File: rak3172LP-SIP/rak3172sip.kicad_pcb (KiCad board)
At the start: 2 copper layers, 46.5 x 29 mm, 46 parts, among them J1 U.FL, J2 Conn_ARM_SWD_TagConnect_TC203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, J4 Conn_01x03_Socket, J5 Conn_01x02_Socket, J6 Conn_01x08_Socket, U1 RAK3172-SIP

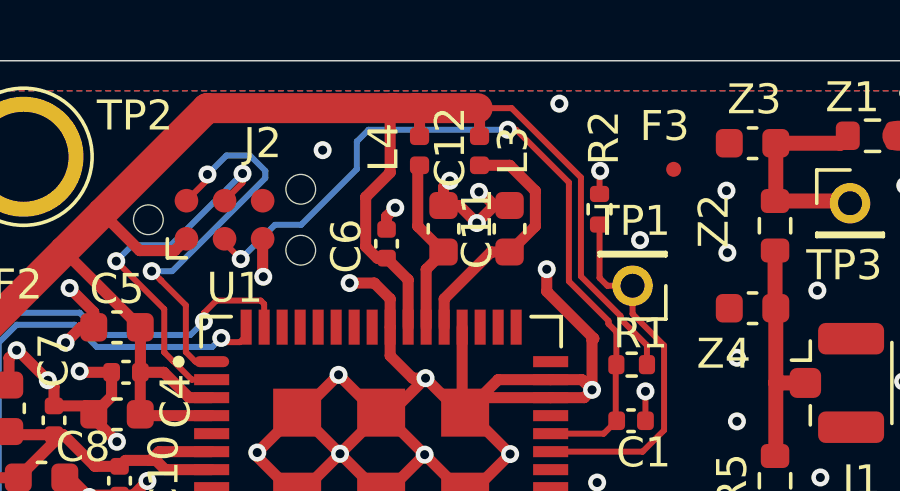
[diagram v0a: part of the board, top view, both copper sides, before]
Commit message: 0v02
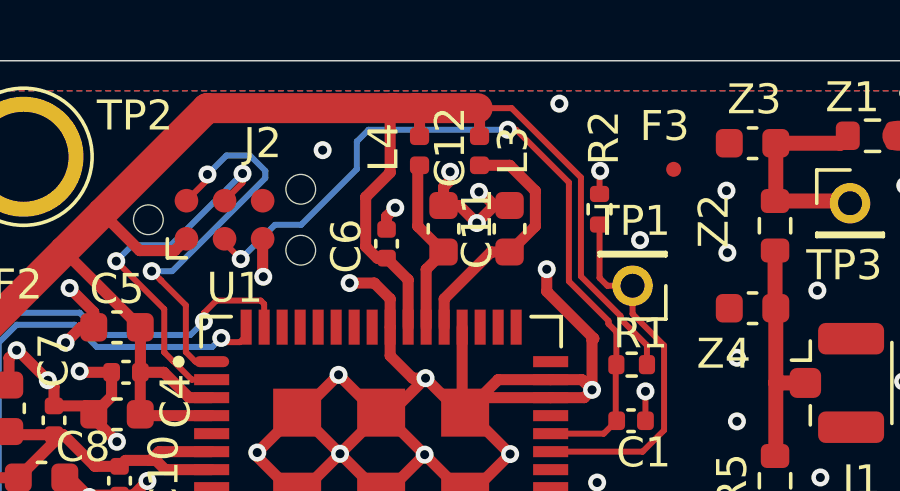
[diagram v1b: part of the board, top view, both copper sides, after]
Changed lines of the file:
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@@
 			(outputformat 1)
 			(mirror no)
-			(drillshape 1)
+			(drillshape 0)
 			(scaleselection 1)
-			(outputdirectory "")
+			(outputdirectory "rak3172_prod/")
 		)
 	)
@@
 		(sheetname "/")
 		(sheetfile "rak3172sip.kicad_sch")
-		(attr smd)
+		(attr smd dnp)
 		(fp_line
 			(start -0.237258 -0.5225)
@@
 		(sheetname "/")
 		(sheetfile "rak3172sip.kicad_sch")
-		(attr smd)
+		(attr smd dnp)
 		(fp_line
 			(start -0.237258 -0.5225)
@@
 			)
 		)
-		(property "Description" "Inductor with ferrite core, small symbol"
+		(property "Description" "FerriteBead Murata MPZ1005S121ETD25"
 			(at 0 0 0)
 			(layer "F.Fab")
@@
 		(sheetname "/")
 		(sheetfile "rak3172sip.kicad_sch")
-		(attr smd)
+		(attr smd dnp)
 		(fp_line
 			(start -0.14058 0.51)
@@
 			)
 		)
-		(property "Description" "Inductor with ferrite core, small symbol"
+		(property "Description" "FerriteBead Murata MPZ1005S121ETD25"
 			(at 0 0 90)
 			(layer "F.Fab")
@@
 			)
 		)
-		(property "Description" "Inductor"
+		(property "Description" "Inductor LQM21DN150M70L"
 			(at 0 0 90)
 			(layer "F.Fab")
@@
 		(sheetname "/")
 		(sheetfile "rak3172sip.kicad_sch")
-		(attr through_hole)
+		(attr through_hole exclude_from_bom)
 		(fp_line
 			(start -1.38 6.46)
@@
 			)
 		)
-		(property "Description" "Inductor with ferrite core, small symbol"
+		(property "Description" "FerriteBead Murata MPZ1005S121ETD25"
 			(at 0 0 90)
 			(layer "F.Fab")
@@
 		(sheetname "/")
 		(sheetfile "rak3172sip.kicad_sch")
-		(attr smd)
+		(attr smd dnp)
 		(fp_line
 			(start -0.14058 0.51)
@@
 			)
 		)
-		(property "Datasheet" ""
+		(property "Datasheet" "https://store.rakwireless.com/products/wisduo-module-rak3172-sip?variant=42482784796870"
 			(at 0 0 0)
 			(layer "F.Fab")
@@
 			)
 		)
-		(property "Description" ""
+		(property "Description" "RAK3172LP-SiP / 8XXMHz for EU868/IN865/RU864  SKU: 305049"
 			(at 0 0 0)
 			(layer "F.Fab")
@@
 		(sheetname "/")
 		(sheetfile "rak3172sip.kicad_sch")
-		(attr through_hole)
+		(attr through_hole exclude_from_bom)
 		(fp_line
 			(start -1.11 -1.11)
@@
 		(sheetname "/")
 		(sheetfile "rak3172sip.kicad_sch")
-		(attr exclude_from_pos_files)
+		(attr exclude_from_pos_files exclude_from_bom)
 		(fp_circle
 			(center 0 0)
@@
 			)
 		)
-		(property "Description" "Light emitting diode"
+		(property "Description" "LED (generic, bright, LowCost)"
 			(at 0 0 0)
 			(layer "F.Fab")
@@
 		(sheetname "/")
 		(sheetfile "rak3172sip.kicad_sch")
-		(attr through_hole)
+		(attr through_hole exclude_from_bom)
 		(fp_line
 			(start -1.38 19.16)
@@
 		(sheetname "/")
 		(sheetfile "rak3172sip.kicad_sch")
-		(attr exclude_from_pos_files)
+		(attr exclude_from_pos_files exclude_from_bom)
 		(fp_circle
 			(center 0 0)
@@
 			)
 		)
-		(property "Description" "coaxial connector (BNC, SMA, SMB, SMC, Cinch/RCA, LEMO, ...)"
+		(property "Description" "U.FL socket (generic)"
 			(at 0 0 0)
 			(unlocked yes)
@@
 		(sheetname "/")
 		(sheetfile "rak3172sip.kicad_sch")
-		(attr smd)
+		(attr smd exclude_from_bom)
 		(fp_rect
 			(start -0.515 -0.94)
@@
 		(sheetname "/")
 		(sheetfile "rak3172sip.kicad_sch")
-		(attr through_hole)
+		(attr through_hole exclude_from_bom)
 		(fp_line
 			(start -1.38 -1.38)
@@
 	)
 	(via
-		(at 99.91 74.5)
+		(at 99.92 74.2)
 		(size 0.6)
 		(drill 0.3)
